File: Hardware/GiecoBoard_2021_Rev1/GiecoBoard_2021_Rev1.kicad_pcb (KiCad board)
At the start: 2 copper layers, 125.7 x 104.1 mm, 57 parts, among them J1 Conn_02x02_Top_Bottom, J10 Conn_02x02_Top_Bottom, J2 Conn_02x02_Top_Bottom, J3 Conn_02x02_Top_Bottom, J4 Conn_02x02_Top_Bottom, J5 Conn_02x02_Top_Bottom, J6 Conn_02x02_Top_Bottom, J7 Conn_02x02_Top_Bottom, J8 Conn_02x02_Top_Bottom, J9 Conn_02x02_Top_Bottom, U1 TM4C129E_Launchpad, U2 OKI

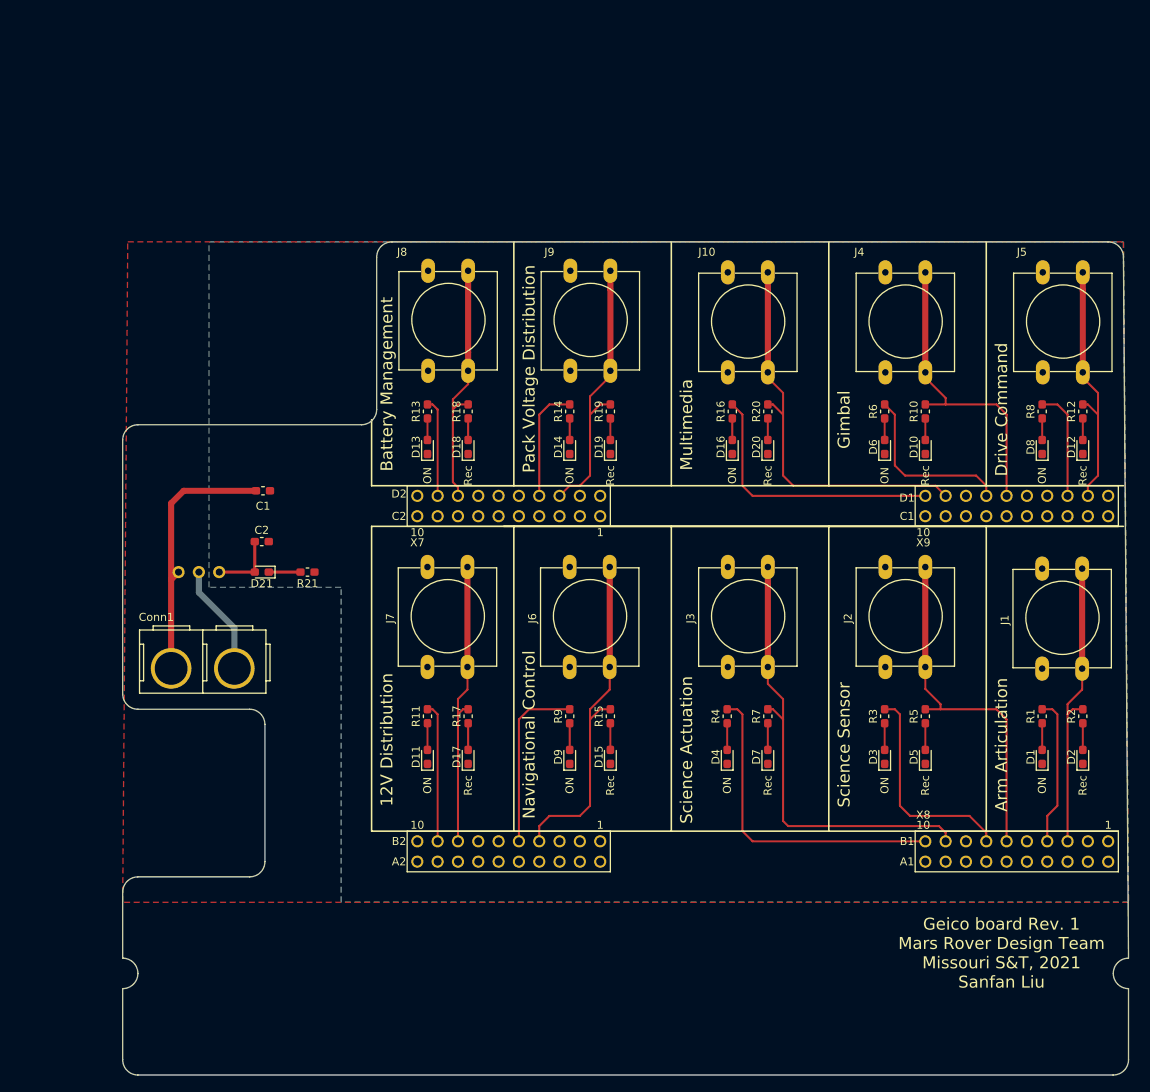
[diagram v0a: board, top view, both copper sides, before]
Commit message: flip tiva and wiring
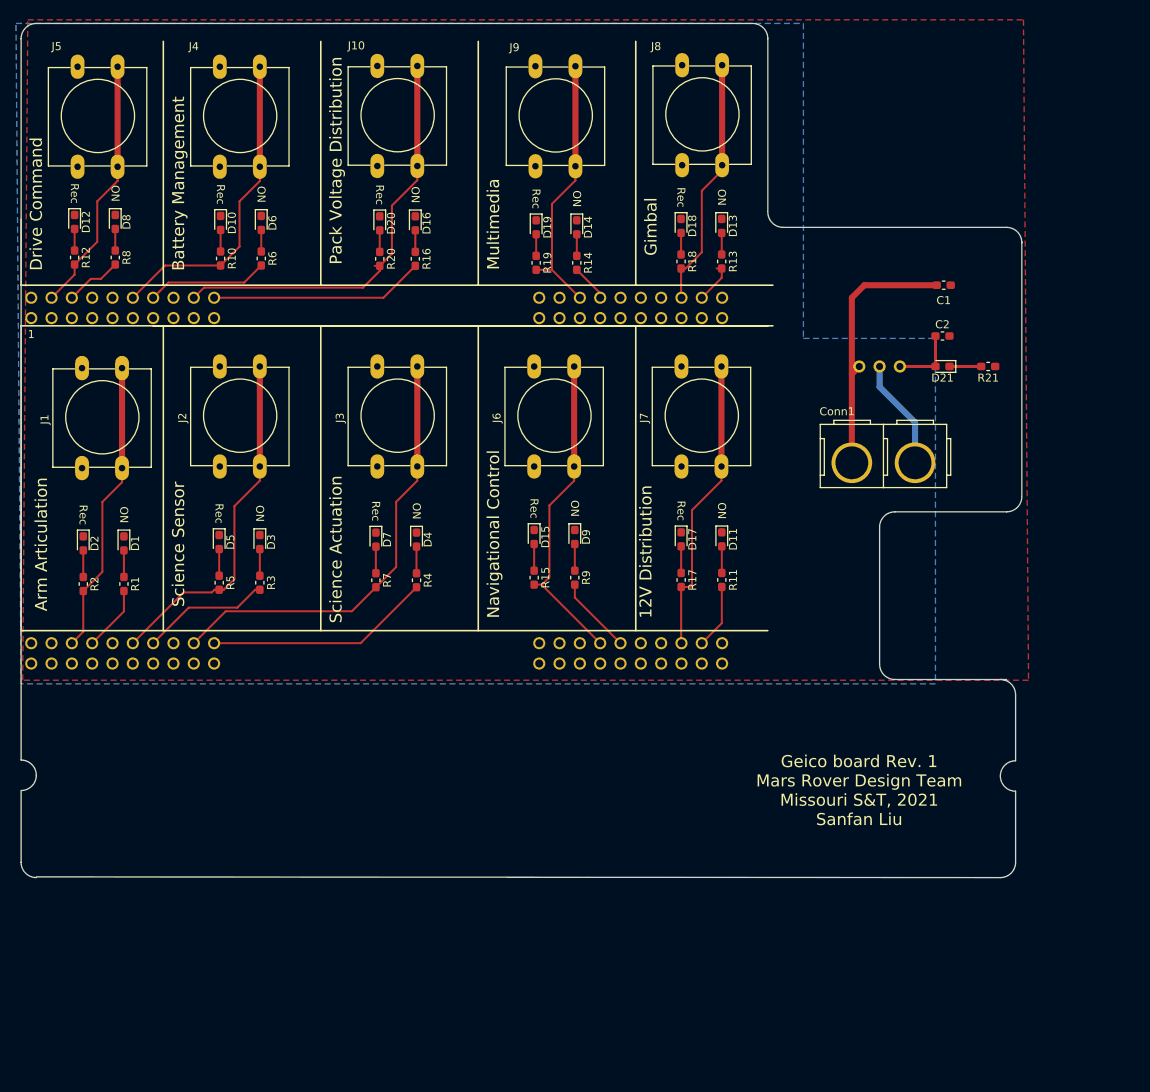
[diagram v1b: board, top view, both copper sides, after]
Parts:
- U1: moved to F.Cu
- moved U1 139.4 mm to (86.4, 112.4), turned to 0 degrees
- moved D12 129.1 mm to (93.1, 55.9), turned to 270 degrees
- moved D2 127.8 mm to (94.1, 96.1), turned to 270 degrees
- moved R12 127.5 mm to (93.1, 60.4), turned to 270 degrees
- moved R2 126.0 mm to (94.1, 101.2), turned to 270 degrees
- moved J5 123.4 mm to (93.4, 49.0)
- moved J1 122.6 mm to (94.0, 86.7)
- moved D8 119.2 mm to (98.1, 55.9), turned to 270 degrees
- moved D1 117.8 mm to (99.2, 96.1), turned to 270 degrees
- moved R8 117.4 mm to (98.1, 60.4), turned to 270 degrees
- moved R1 116.0 mm to (99.2, 101.2), turned to 270 degrees
- moved D10 92.4 mm to (111.3, 56.1), turned to 270 degrees
- moved D5 92.3 mm to (111.1, 95.9), turned to 270 degrees
- moved R10 90.1 mm to (111.3, 60.5), turned to 270 degrees
- moved R5 89.8 mm to (111.1, 101.0), turned to 270 degrees
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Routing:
- net REC_LED_NavigationalControl: track 22.1 -> 9.69 mm
- net REC_LED_ScienceActuation: track 40.2 -> 28.2 mm
- net REC_LED_ScienceSensor: track 26.9 -> 16.1 mm
- net REC_LED_ArmArticulation: track 18.6 -> 8.17 mm
- net REC_LED_PackVoltageDistribution: track 14.5 -> 4.70 mm
- net REC_LED_12VDistribution: track 17.4 -> 8.07 mm
- net REC_LED_Multimedia: track 34.1 -> 26.8 mm
- net REC_LED_BatteryManagement: track 12.3 -> 5.32 mm
- net REC_LED_DriveCommand: track 13.9 -> 7.14 mm
- net REC_LED_Gimbal: track 21.9 -> 15.2 mm
- net Send_NavigationalControl: track 43.2 -> 40.3 mm
- net Send_Multimedia: track 50.0 -> 52.8 mm
- net Send_ScienceActuation: track 57.0 -> 55.4 mm
- net Send_12VDistribution: track 36.3 -> 37.5 mm
- net Send_Gimbal: track 38.4 -> 39.5 mm
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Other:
- board size 125.7 x 104.1 mm -> 125.1 x 106.8 mm
